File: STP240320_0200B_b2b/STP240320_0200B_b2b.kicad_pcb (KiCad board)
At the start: 2 copper layers, 6.1 x 11.2 mm, 2 parts, among them J1 Conn_02x08_Odd_Even

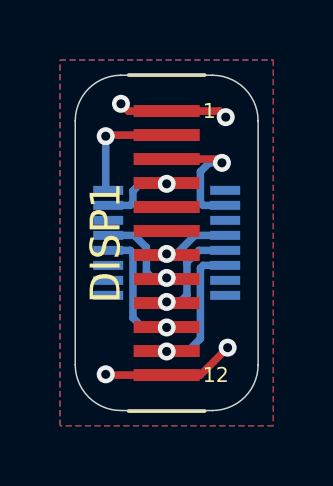
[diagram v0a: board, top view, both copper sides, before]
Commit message: ci: add CI (#1)
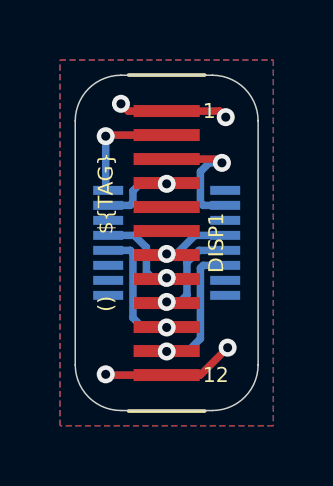
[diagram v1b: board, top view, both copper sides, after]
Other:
- board text added: "${TAG}"
- board text added: "(${REVISION})"
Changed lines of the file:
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@@
     )
   )
+  (property "DATE" "YYYY-MM-DD HH:MM:SS")
+  (property "REVISION" "REVISION")
+  (property "TAG" "TAG")
   (net 0 "")
   (net 1 "GND")
@@
     (at 116.332 83.9978)
     (attr through_hole)
-    (fp_text reference "DISP1" (at -2.032 4.3942 90) (layer "F.SilkS")
-      (effects (font (size 1 1) (thickness 0.15)))
+    (fp_text reference "DISP1" (at 1.651 4.3942 270) (layer "F.SilkS")
+      (effects (font (size 0.5 0.5) (thickness 0.1)))
     )
     (fp_text value "STP240320_0200B" (at -4.064 3.8862 90) (layer "F.Fab")
@@
   (gr_line (start 119.38 92.456) (end 119.38 84.328) (layer "Edge.Cuts") (width 0.05))
   (gr_arc (start 113.284 84.328) (mid 113.730369 83.250369) (end 114.808 82.804) (layer "Edge.Cuts") (width 0.05))
+  (gr_text "${TAG}" (at 114.3 86.741 90) (layer "F.SilkS")
+    (effects (font (size 0.5 0.5) (thickness 0.1)))
+  )
+  (gr_text "(${REVISION})" (at 114.3 90.424 90) (layer "F.SilkS")
+    (effects (font (size 0.5 0.5) (thickness 0.1)))
+  )
   (segment (start 116.332 83.9978) (end 118.0973 83.9978) (width 0.25) (layer "F.Cu") (net 1))
   (segment (start 115.0493 83.9978) (end 114.808 83.7565) (width 0.25) (layer "F.Cu") (net 1))
